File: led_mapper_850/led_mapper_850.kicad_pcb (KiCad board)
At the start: 2 copper layers, 530 parts, among them J1 Conn_02x12_Top_Bottom

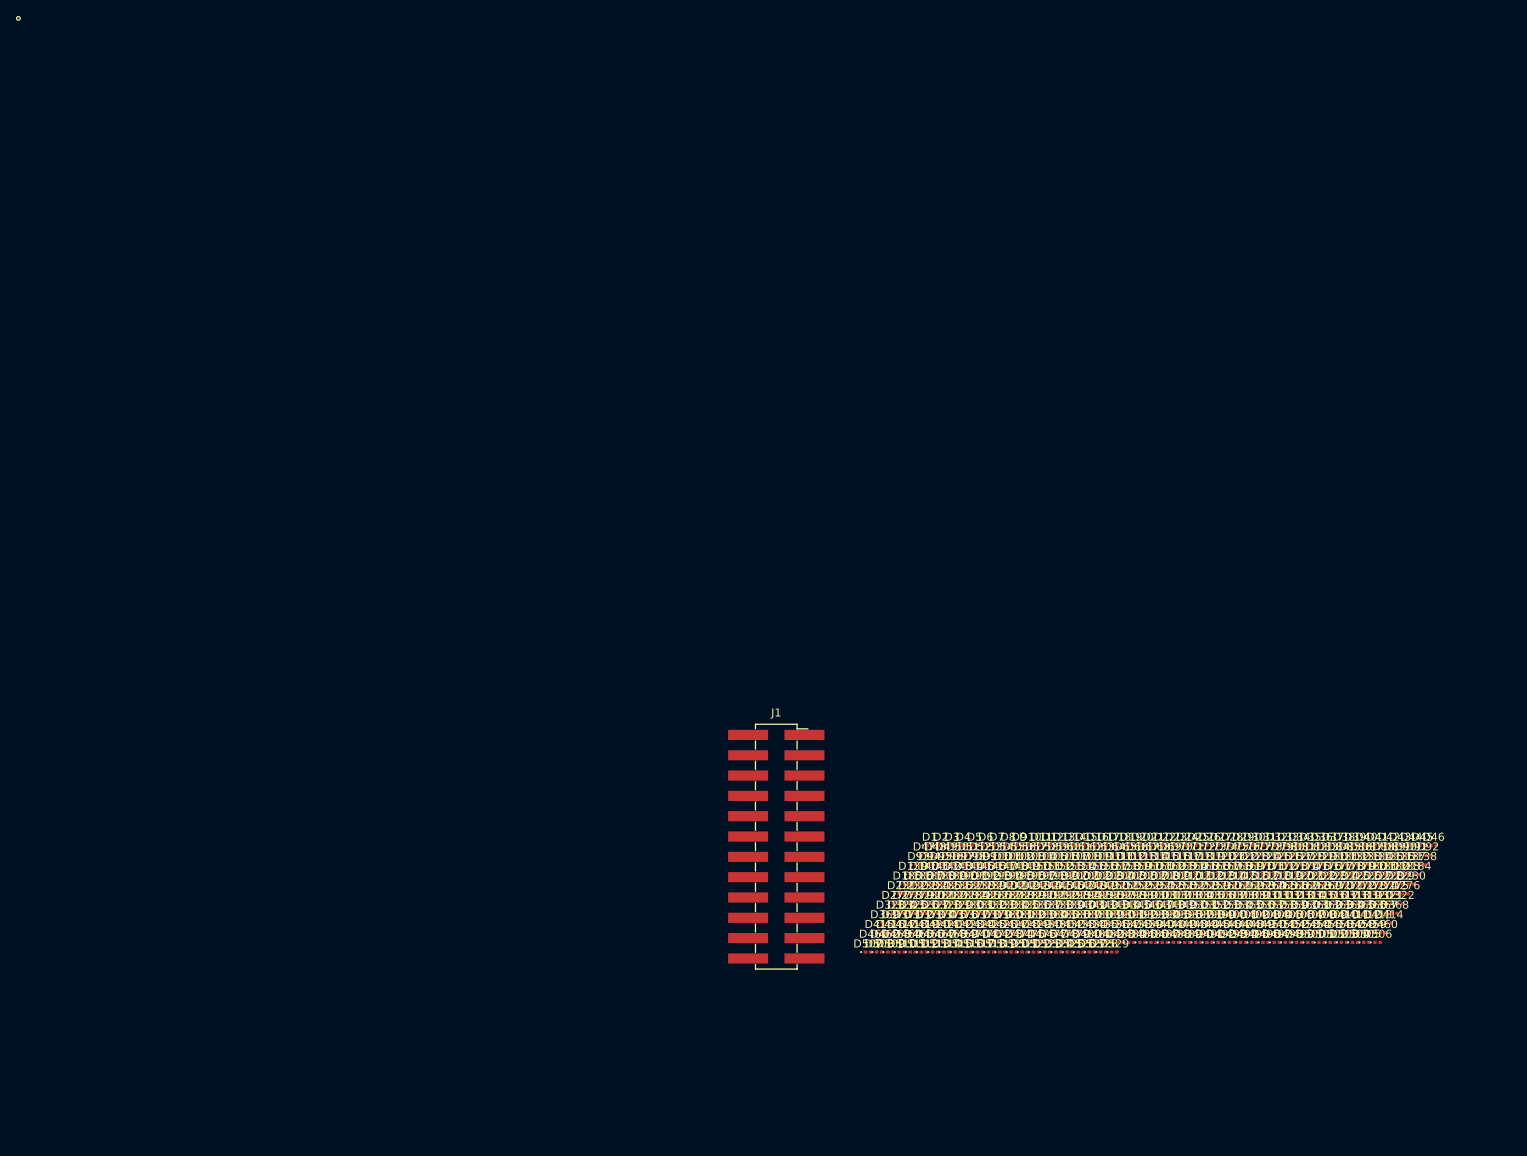
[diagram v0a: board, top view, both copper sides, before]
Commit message: place vias
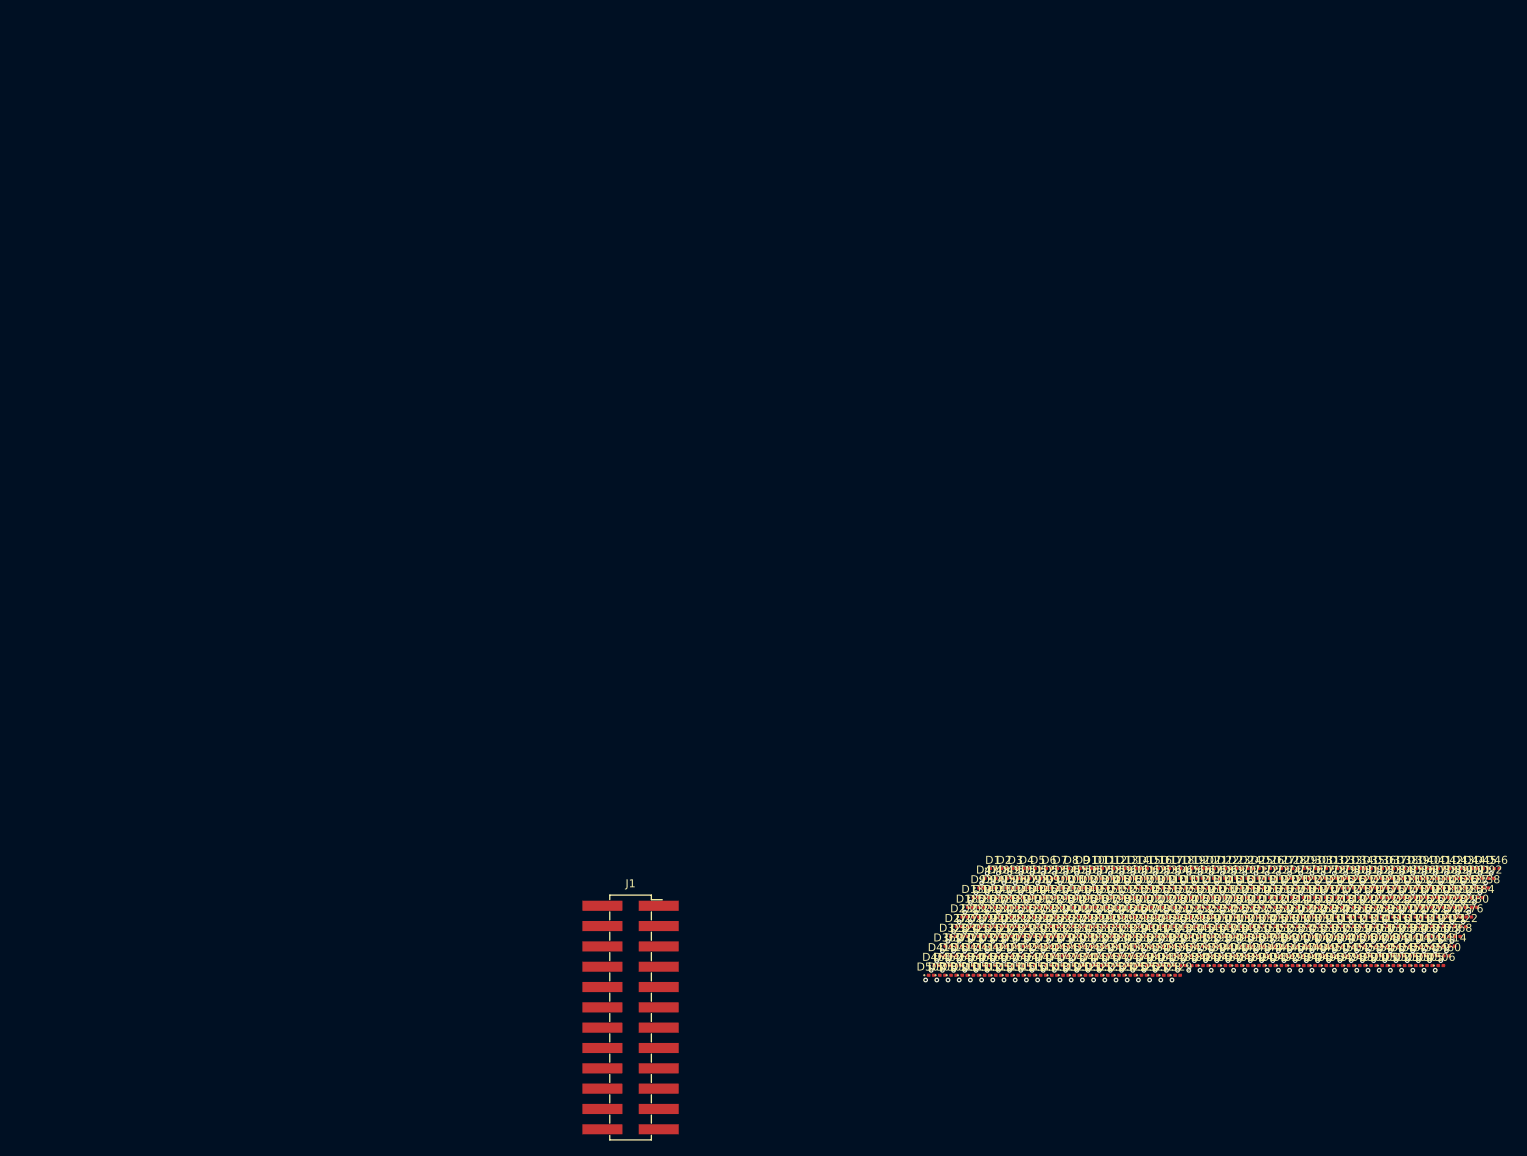
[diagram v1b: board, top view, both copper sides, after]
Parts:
- moved J1 28.1 mm to (76.5, 124.9)
- moved D10 8.41 mm to (134.4, 106.3)
- moved D102 8.41 mm to (133.0, 108.7)
- moved D103 8.41 mm to (134.4, 108.7)
- moved D104 8.41 mm to (135.8, 108.7)
- moved D106 8.41 mm to (138.6, 108.7)
- moved D107 8.41 mm to (140.0, 108.7)
- moved D108 8.41 mm to (141.4, 108.7)
- moved D109 8.41 mm to (142.8, 108.7)
- moved D11 8.41 mm to (135.8, 106.3)
- moved D111 8.41 mm to (145.6, 108.7)
- moved D112 8.41 mm to (147.0, 108.7)
- moved D113 8.41 mm to (148.4, 108.7)
- moved D114 8.41 mm to (149.8, 108.7)
- moved D116 8.41 mm to (152.6, 108.7)
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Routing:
- net /P24: vias 0 -> 23
- net /P23: vias 0 -> 23
- net /P22: vias 0 -> 23
- net /P21: vias 0 -> 23
- net /P20: vias 0 -> 23
- net /P19: vias 0 -> 23
- net /P18: vias 0 -> 23
- net /P17: vias 0 -> 23
- net /P16: vias 0 -> 23
- net /P15: vias 0 -> 23
- net /P14: vias 0 -> 23
- net /P13: vias 0 -> 23
- net /P12: vias 0 -> 23
- net /P11: vias 0 -> 23
- net /P10: vias 0 -> 23
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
